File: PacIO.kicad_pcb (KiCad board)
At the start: 2 copper layers, 44.4 x 50.8 mm, 15 parts, among them J1 PacMan_Connector, J2 E-ink Display, J3 Charge LED

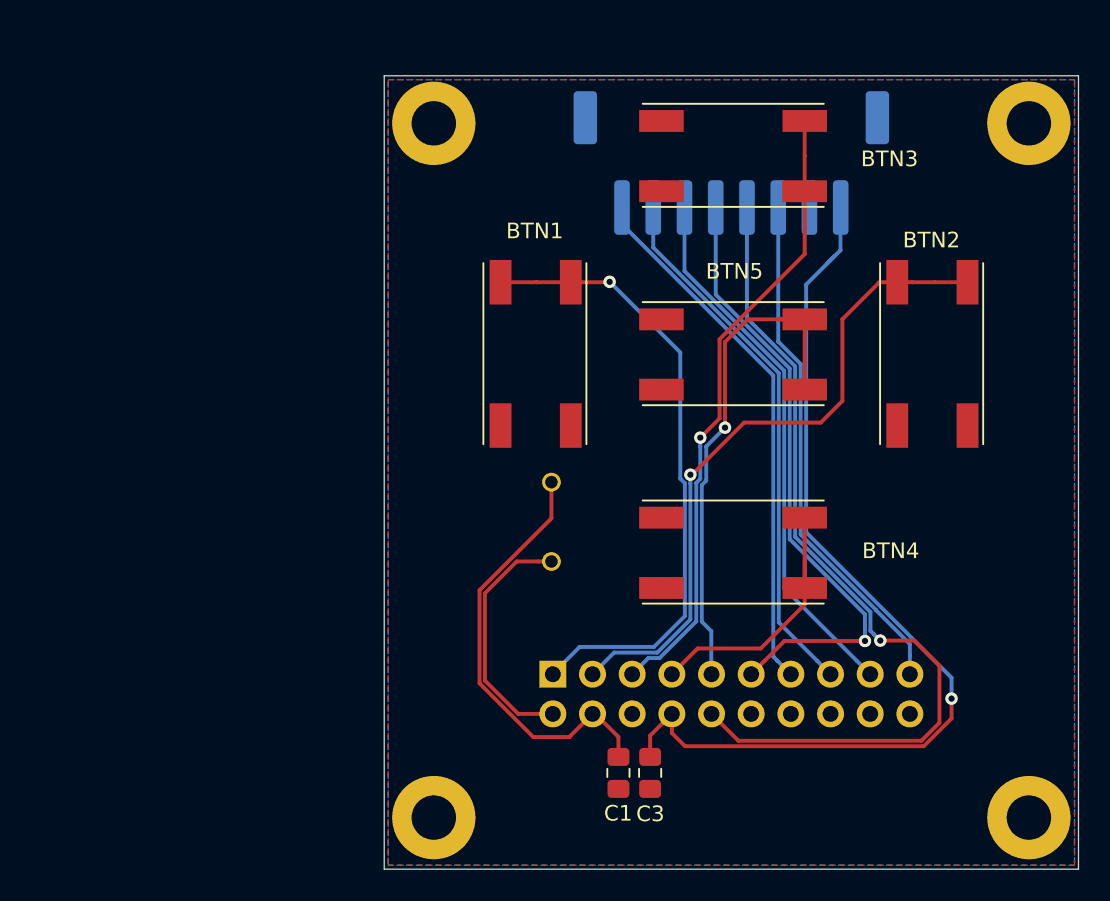
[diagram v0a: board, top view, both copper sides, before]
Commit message: New Origin
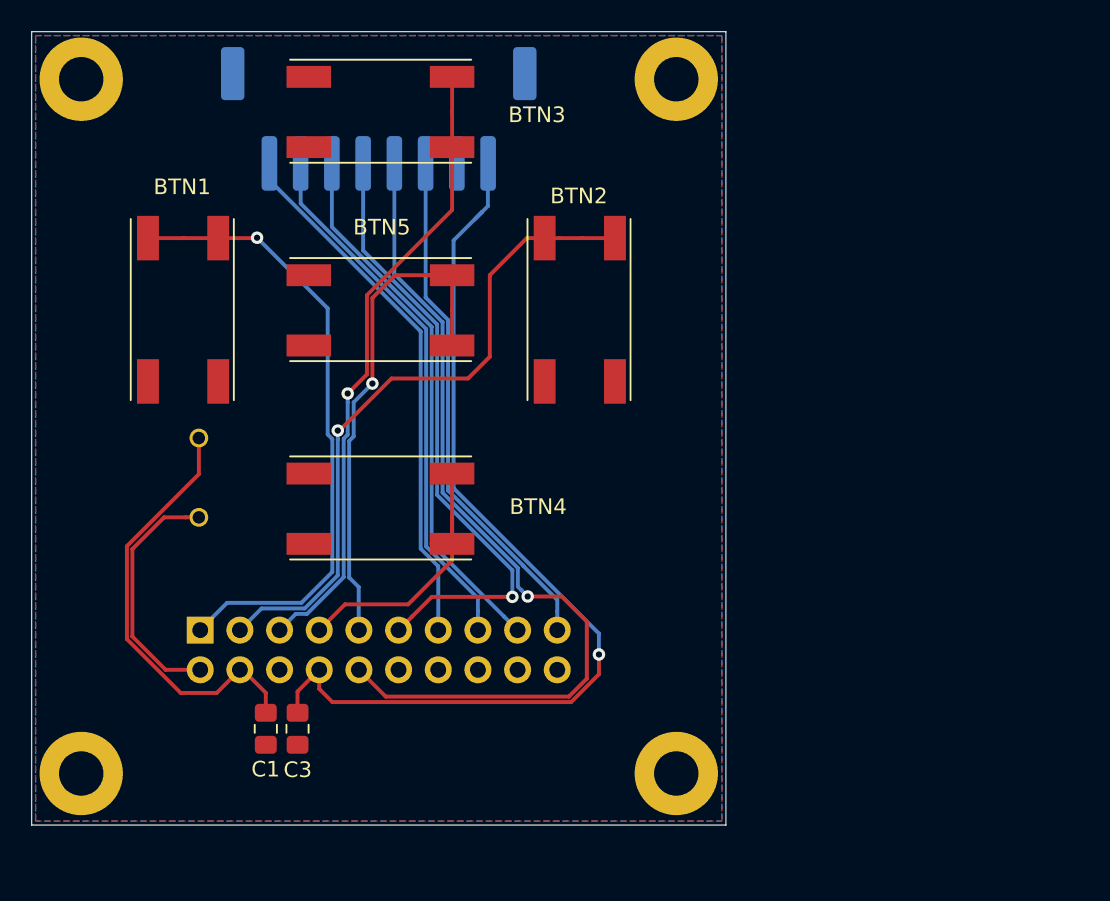
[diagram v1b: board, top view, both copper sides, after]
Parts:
- moved BTN1 22.8 mm to (118.4, 95.5)
- moved BTN2 22.8 mm to (143.8, 95.5)
- moved C1 22.8 mm to (123.7, 122.3)
- moved C3 22.8 mm to (125.8, 122.3)
- moved J2 22.8 mm to (131.0, 83.3)
- moved LOGO2 22.8 mm to (132.5, 106.3)
- moved H1 22.8 mm to (111.9, 80.7)
- moved H4 22.8 mm to (111.9, 125.2)
- moved J1 22.8 mm to (119.5, 116.0)
- moved J3 22.8 mm to (119.4, 106.3)
- moved BTN3 22.8 mm to (131.1, 82.8)
- moved BTN4 22.8 mm to (131.1, 108.2)
- moved BTN5 22.8 mm to (131.1, 95.5)
- moved H2 22.8 mm to (150.0, 80.7)
- moved H3 22.8 mm to (150.0, 125.2)
